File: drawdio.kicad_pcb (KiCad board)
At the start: 2 copper layers, 47 x 17 mm, 12 parts, among them P1 CONN_2, P2 SPK, Q1 BC558, Q2 BC547, U1 LM555N

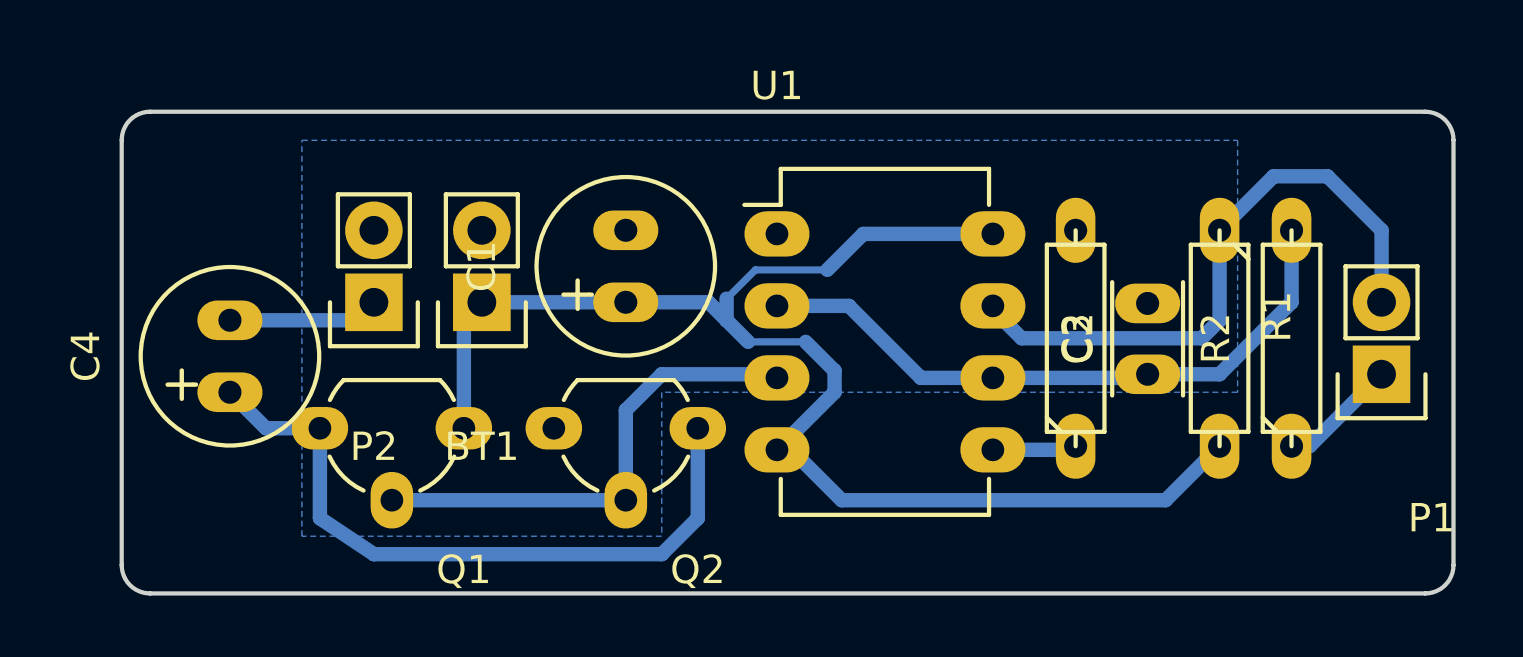
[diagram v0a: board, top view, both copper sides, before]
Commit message: V0.2
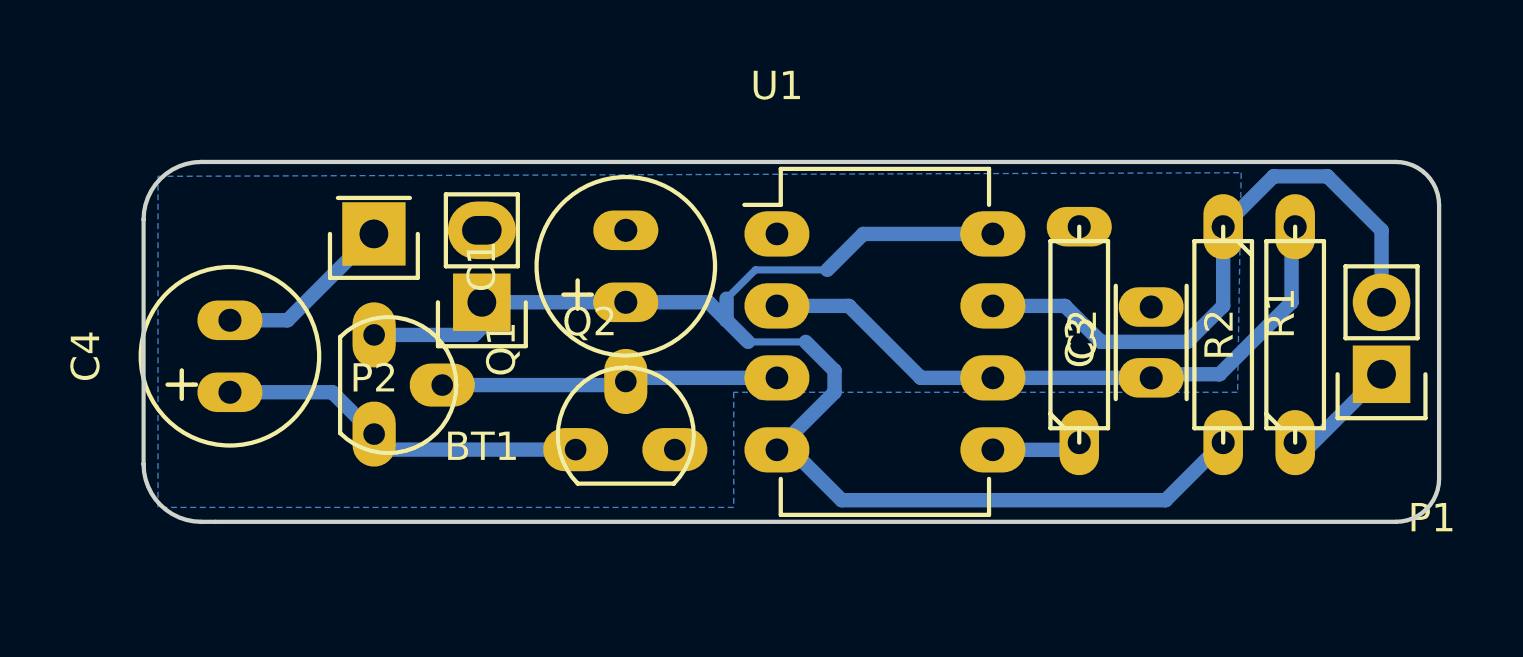
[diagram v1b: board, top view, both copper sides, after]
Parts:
- P2: value SPK -> CONN_01X01; footprint Pin_Headers:Pin_Header_Straight_1x02 -> Pin_Headers:Pin_Header_Straight_1x01
- Q1, Q2: footprint Housings_TO-92:TO-92_Molded_Wide_Oval -> drawdio:TO-92_JorFru_compact
- moved Q1 3.86 mm to (89.4, 87.4), turned to 270 degrees
- moved Q2 3.82 mm to (96.5, 90.4), turned to 0 degrees
- moved P2 2.41 mm to (88.9, 83.3)
- moved R1 0.18 mm to (121.4, 86.9)
- moved C2 0.18 mm to (113.8, 86.9)
- moved R2 0.18 mm to (118.9, 86.9)
- moved C3 0.18 mm to (116.3, 88.4)
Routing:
- net Net-(C4-Pad1): track 23.7 -> 13.0 mm
- net Net-(Q1-Pad2): track 17.3 -> 13.3 mm
- net VCC: track 50.3 -> 51.7 mm
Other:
- board size 47 x 17 mm -> 45.7 x 12.7 mm
